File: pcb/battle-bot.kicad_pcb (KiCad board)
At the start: 4 copper layers, 99.2 x 51.2 mm, 27 parts, among them U1 TPS5430DDA, U2 STM32G474VETx

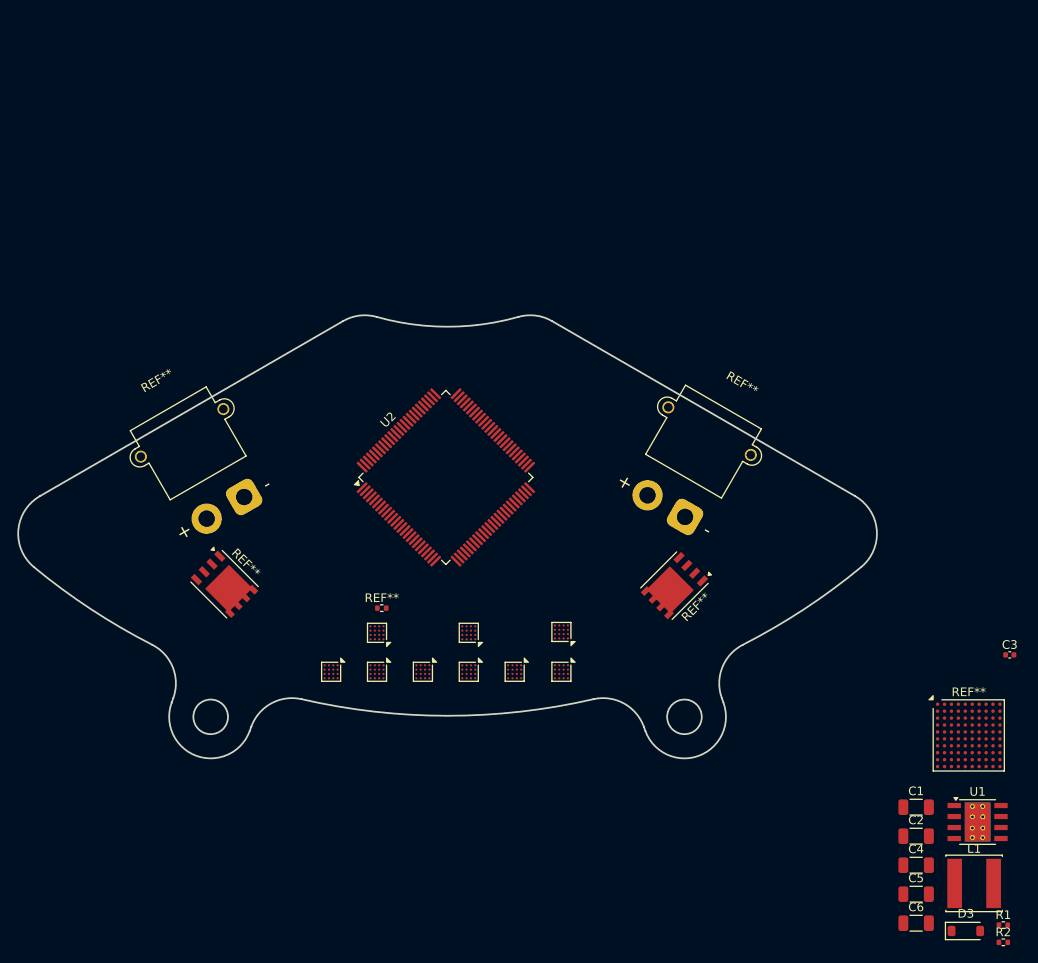
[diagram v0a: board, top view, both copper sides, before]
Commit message: Finish drivers
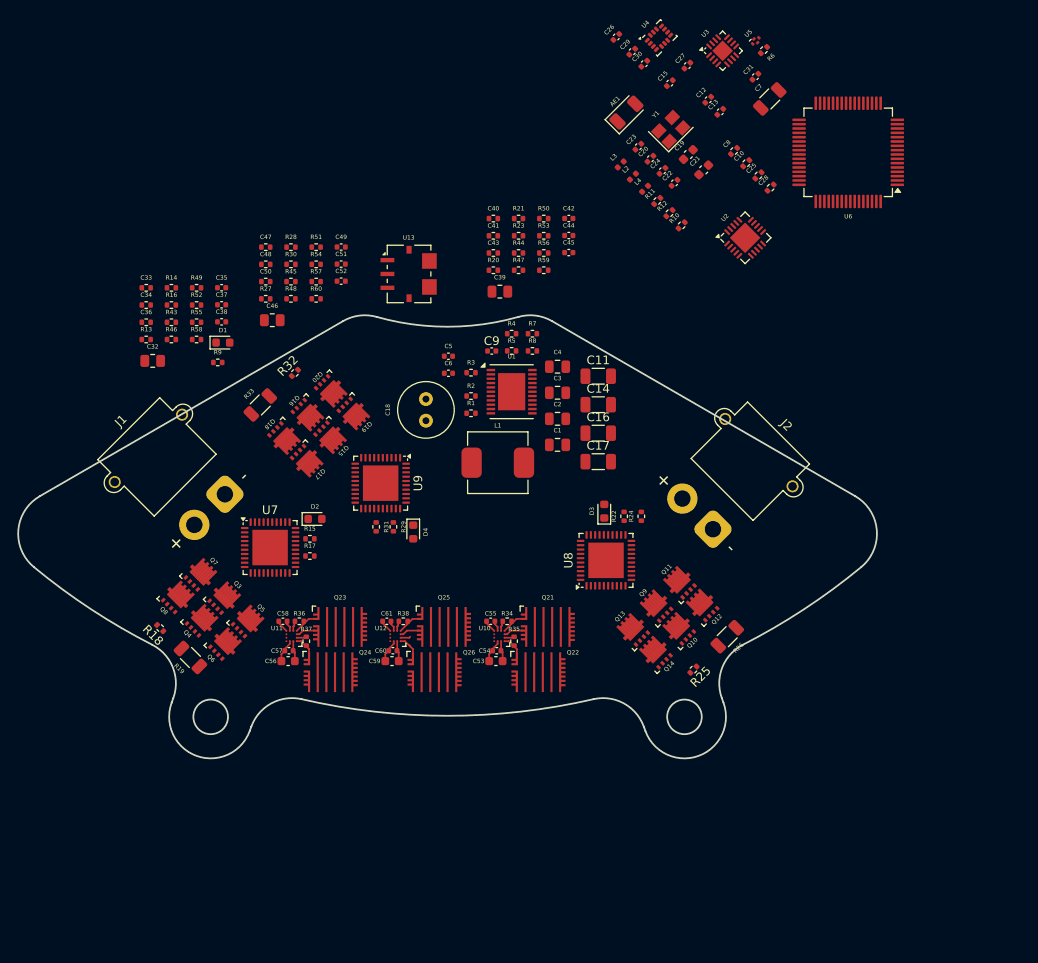
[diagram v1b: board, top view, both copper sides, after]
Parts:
- removed REF** (x9): BGA-16_1.92x1.92mm_Layout4x4_P0.5mm, Package_BGA:BGA-16_1.92x1.92mm_Layout4x4_P0.5mm
- removed REF** (x2): AMASS_XT30PW-M_1x02_P2.50mm_Horizontal, Connector_AMASS:AMASS_XT30PW-M_1x02_P2.50mm_Horizontal
- removed REF**: TFBGA-100_8x8mm_Layout10x10_P0.8mm, Package_BGA:TFBGA-100_8x8mm_Layout10x10_P0.8mm
- removed REF** (x2): PowerPAK_SO-8_Single, Package_SO:PowerPAK_SO-8_Single
- removed REF**: R_0402_1005Metric, Resistor_SMD:R_0402_1005Metric
- added AE1: Antenna, RF_Antenna:Johanson_2450AT18x100, F.Cu at (120.8, 7.26)
- added C10: 100n, Resistor_SMD:R_0402_1005Metric, F.Cu at (134.7, 13.1)
- added C11: 47u, Capacitor_SMD:C_1206_3216Metric, F.Cu at (117.6, 37.7)
- added C12: 10n, Capacitor_SMD:C_0402_1005Metric, F.Cu at (130.3, 5.78)
- added C13: 33n, Capacitor_SMD:C_0402_1005Metric, F.Cu at (131.7, 7.17)
- added C14: 47u, Capacitor_SMD:C_1206_3216Metric, F.Cu at (117.6, 41.0)
- added C15: 1n, Capacitor_SMD:C_0402_1005Metric, F.Cu at (125.9, 3.86)
- added C16: 47u, Capacitor_SMD:C_1206_3216Metric, F.Cu at (117.6, 44.3)
- added C17: 47u, Capacitor_SMD:C_1206_3216Metric, F.Cu at (117.6, 47.6)
- added C18: 220u, Capacitor_THT:C_Radial_D6.3mm_H7.0mm_P2.50mm, F.Cu at (97.7, 42.8)
- added C19: 2n2, Capacitor_SMD:C_0603_1608Metric, F.Cu at (128.0, 12.1)
- added C20: 12p, Capacitor_SMD:C_0402_1005Metric, F.Cu at (123.6, 12.6)
- added C21: 4p7, Capacitor_SMD:C_0603_1608Metric, F.Cu at (129.8, 13.9)
- added C22: 1p5, Capacitor_SMD:C_0402_1005Metric, F.Cu at (126.4, 15.4)
- added C23: 12p, Capacitor_SMD:C_0402_1005Metric, F.Cu at (122.2, 11.2)
- added C24: 1p, Capacitor_SMD:C_0402_1005Metric, F.Cu at (125.0, 14.0)
- added C25: 10u, Resistor_SMD:R_0402_1005Metric, F.Cu at (136.1, 14.5)
- added C26: 4u7, Capacitor_SMD:C_0402_1005Metric, F.Cu at (119.7, -1.48)
- added C27: 10n, Capacitor_SMD:C_0402_1005Metric, F.Cu at (127.9, 1.83)
- added C28: 220p, Resistor_SMD:R_0402_1005Metric, F.Cu at (137.5, 15.9)
- added C29: 100n, Capacitor_SMD:C_0402_1005Metric, F.Cu at (121.5, 0.22)
- added C30: 100n, Capacitor_SMD:C_0402_1005Metric, F.Cu at (122.9, 1.61)
- added C31: 0p3, Capacitor_SMD:C_0402_1005Metric, F.Cu at (135.8, 3.11)
- added C32: 22u, Resistor_SMD:R_0805_2012Metric, F.Cu at (66.1, 35.9)
- added C33: 1u, Resistor_SMD:R_0402_1005Metric, F.Cu at (65.4, 27.5)
- added C34: 1u, Resistor_SMD:R_0402_1005Metric, F.Cu at (65.4, 29.5)
- added C35: 100n, Capacitor_SMD:C_0402_1005Metric, F.Cu at (74.1, 27.5)
- added C36: 1u, Resistor_SMD:R_0402_1005Metric, F.Cu at (65.4, 31.5)
- added C37: 47n, Capacitor_SMD:C_0402_1005Metric, F.Cu at (74.1, 29.5)
- added C38: 100n, Capacitor_SMD:C_0402_1005Metric, F.Cu at (74.1, 31.4)
- added C39: 22u, Resistor_SMD:R_0805_2012Metric, F.Cu at (106.2, 27.9)
- added C40: 1u, Resistor_SMD:R_0402_1005Metric, F.Cu at (105.5, 19.5)
- added C41: 1u, Resistor_SMD:R_0402_1005Metric, F.Cu at (105.5, 21.5)
- added C42: 100n, Capacitor_SMD:C_0402_1005Metric, F.Cu at (114.2, 19.5)
- added C43: 1u, Resistor_SMD:R_0402_1005Metric, F.Cu at (105.5, 23.5)
- added C44: 47n, Capacitor_SMD:C_0402_1005Metric, F.Cu at (114.2, 21.5)
- added C45: 100n, Capacitor_SMD:C_0402_1005Metric, F.Cu at (114.2, 23.4)
- added C46: 22u, Resistor_SMD:R_0805_2012Metric, F.Cu at (80.0, 31.2)
- added C47: 1u, Resistor_SMD:R_0402_1005Metric, F.Cu at (79.2, 22.8)
- added C48: 1u, Resistor_SMD:R_0402_1005Metric, F.Cu at (79.2, 24.8)
- added C49: 100n, Capacitor_SMD:C_0402_1005Metric, F.Cu at (87.9, 22.8)
- added C50: 1u, Resistor_SMD:R_0402_1005Metric, F.Cu at (79.2, 26.8)
- added C51: 47n, Capacitor_SMD:C_0402_1005Metric, F.Cu at (87.9, 24.8)
- added C52: 100n, Capacitor_SMD:C_0402_1005Metric, F.Cu at (87.9, 26.7)
- added C53: 10u, Capacitor_SMD:C_0603_1608Metric, F.Cu at (105.8, 70.6)
- added C54: 100n, Capacitor_SMD:C_0402_1005Metric, F.Cu at (105.9, 69.4)
- added C55: 220n, Capacitor_SMD:C_0402_1005Metric, F.Cu at (105.2, 66.0)
- added C56: 10u, Capacitor_SMD:C_0603_1608Metric, F.Cu at (81.8, 70.6)
- added C57: 100n, Capacitor_SMD:C_0402_1005Metric, F.Cu at (81.9, 69.4)
- added C58: 220n, Capacitor_SMD:C_0402_1005Metric, F.Cu at (81.2, 66.0)
- added C59: 10u, Capacitor_SMD:C_0603_1608Metric, F.Cu at (93.8, 70.6)
- added C60: 100n, Capacitor_SMD:C_0402_1005Metric, F.Cu at (93.9, 69.4)
- added C61: 220n, Capacitor_SMD:C_0402_1005Metric, F.Cu at (93.2, 66.0)
- added C7: 100u, Resistor_SMD:R_1206_3216Metric, F.Cu at (137.4, 5.69)
- added C8: 10u, Resistor_SMD:R_0402_1005Metric, F.Cu at (133.3, 11.7)
- added C9: 100n, Capacitor_SMD:C_0402_1005Metric, F.Cu at (105.3, 34.8)
- added D1: LEDG, LED_SMD:LED_0603_1608Metric, F.Cu at (74.2, 33.8)
- added D2: LEDR, LED_SMD:LED_0603_1608Metric, F.Cu at (84.9, 54.2)
- added D4: LEDR, LED_SMD:LED_0603_1608Metric, F.Cu at (96.2, 55.7)
- added J1: Conn_01x02_Pin, Connector_AMASS:AMASS_XT30PW-M_1x02_P2.50mm_Horizontal, F.Cu at (74.5, 51.3)
- added J2: Conn_01x02_Pin, Connector_AMASS:AMASS_XT30PW-M_1x02_P2.50mm_Horizontal, F.Cu at (130.9, 55.4)
- added L2: 2n7, Inductor_SMD:L_0402_1005Metric, F.Cu at (121.6, 14.7)
- added L3: 8n2, Inductor_SMD:L_0402_1005Metric, F.Cu at (120.2, 13.3)
- added L4: 3n9, Inductor_SMD:L_0402_1005Metric, F.Cu at (123.0, 16.1)
- added Q10: AON7544, User_Footprints:DFN3x3A_8L_EP1_P, F.Cu at (127.0, 66.9)
- added Q11: AON7544, User_Footprints:DFN3x3A_8L_EP1_P, F.Cu at (127.1, 61.6)
- added Q12: AON7544, User_Footprints:DFN3x3A_8L_EP1_P, F.Cu at (129.7, 64.2)
- added Q13: AON7544, User_Footprints:DFN3x3A_8L_EP1_P, F.Cu at (121.7, 67.0)
- added Q14: AON7544, User_Footprints:DFN3x3A_8L_EP1_P, F.Cu at (124.3, 69.6)
- added Q15: AON7544, User_Footprints:DFN3x3A_8L_EP1_P, F.Cu at (86.6, 44.8)
- added Q16: AON7544, User_Footprints:DFN3x3A_8L_EP1_P, F.Cu at (84.0, 42.1)
- added Q17: AON7544, User_Footprints:DFN3x3A_8L_EP1_P, F.Cu at (83.9, 47.5)
- added Q18: AON7544, User_Footprints:DFN3x3A_8L_EP1_P, F.Cu at (81.3, 44.8)
- added Q19: AON7544, User_Footprints:DFN3x3A_8L_EP1_P, F.Cu at (89.3, 42.0)
- added Q20: AON7544, User_Footprints:DFN3x3A_8L_EP1_P, F.Cu at (86.7, 39.4)
- added Q21: GANE3R9, User_Footprints:GANE3R9, F.Cu at (111.8, 66.7)
- added Q22: GANE3R9, User_Footprints:GANE3R9, F.Cu at (110.7, 71.9)
- added Q23: GANE3R9, User_Footprints:GANE3R9, F.Cu at (87.8, 66.7)
- added Q24: GANE3R9, User_Footprints:GANE3R9, F.Cu at (86.7, 71.9)
- added Q25: GANE3R9, User_Footprints:GANE3R9, F.Cu at (99.8, 66.7)
- added Q26: GANE3R9, User_Footprints:GANE3R9, F.Cu at (98.7, 71.9)
- added Q3: AON7544, User_Footprints:DFN3x3A_8L_EP1_P, F.Cu at (74.4, 63.4)
- added Q4: AON7544, User_Footprints:DFN3x3A_8L_EP1_P, F.Cu at (71.8, 66.0)
- added Q5: AON7544, User_Footprints:DFN3x3A_8L_EP1_P, F.Cu at (77.1, 66.1)
- added Q6: AON7544, User_Footprints:DFN3x3A_8L_EP1_P, F.Cu at (74.5, 68.7)
- added Q7: AON7544, User_Footprints:DFN3x3A_8L_EP1_P, F.Cu at (71.7, 60.7)
- added Q8: AON7544, User_Footprints:DFN3x3A_8L_EP1_P, F.Cu at (69.0, 63.3)
- added Q9: AON7544, User_Footprints:DFN3x3A_8L_EP1_P, F.Cu at (124.4, 64.3)
- added R10: 1k, Resistor_SMD:R_0402_1005Metric, F.Cu at (127.2, 20.3)
- added R11: 1k, Resistor_SMD:R_0402_1005Metric, F.Cu at (124.4, 17.5)
- added R12: 22k, Resistor_SMD:R_0402_1005Metric, F.Cu at (125.8, 18.9)
- added R13: 47k, Resistor_SMD:R_0402_1005Metric, F.Cu at (65.4, 33.5)
- added R14: 1k, Resistor_SMD:R_0402_1005Metric, F.Cu at (68.3, 27.5)
- added R15: 510k, Resistor_SMD:R_0402_1005Metric, F.Cu at (84.3, 56.5)
- added R16: 47k, Resistor_SMD:R_0402_1005Metric, F.Cu at (68.3, 29.5)
- added R17: 510k, Resistor_SMD:R_0402_1005Metric, F.Cu at (84.3, 58.5)
- added R18: R, Resistor_SMD:R_0402_1005Metric, F.Cu at (67.0, 66.8)
- added R19: 2m, Resistor_SMD:R_1206_3216Metric, F.Cu at (70.5, 70.2)
- added R20: 47k, Resistor_SMD:R_0402_1005Metric, F.Cu at (105.5, 25.5)
- added R21: 1k, Resistor_SMD:R_0402_1005Metric, F.Cu at (108.4, 19.5)
- added R22: 510k, Resistor_SMD:R_0402_1005Metric, F.Cu at (120.6, 53.9)
- added R23: 47k, Resistor_SMD:R_0402_1005Metric, F.Cu at (108.4, 21.5)
- added R24: 510k, Resistor_SMD:R_0402_1005Metric, F.Cu at (122.6, 53.9)
- added R25: R, Resistor_SMD:R_0402_1005Metric, F.Cu at (128.6, 71.6)
- added R26: 2m, Resistor_SMD:R_1206_3216Metric, F.Cu at (132.5, 67.8)
- added R27: 47k, Resistor_SMD:R_0402_1005Metric, F.Cu at (79.2, 28.8)
- added R28: 1k, Resistor_SMD:R_0402_1005Metric, F.Cu at (82.1, 22.8)
- added R29: 510k, Resistor_SMD:R_0402_1005Metric, F.Cu at (93.9, 55.1)
- added R3: 100k, Resistor_SMD:R_0402_1005Metric, F.Cu at (102.9, 37.3)
- added R30: 47k, Resistor_SMD:R_0402_1005Metric, F.Cu at (82.1, 24.8)
- added R31: 510k, Resistor_SMD:R_0402_1005Metric, F.Cu at (92.0, 55.1)
- added R32: 10R, Resistor_SMD:R_0402_1005Metric, F.Cu at (82.6, 37.3)
- added R33: 2m, Resistor_SMD:R_1206_3216Metric, F.Cu at (78.6, 41.0)
- added R34: 10R, Resistor_SMD:R_0402_1005Metric, F.Cu at (107.1, 66.0)
- added R35: 10R, Resistor_SMD:R_0402_1005Metric, F.Cu at (107.9, 68.3)
- added R36: 10R, Resistor_SMD:R_0402_1005Metric, F.Cu at (83.1, 66.0)
- added R37: 10R, Resistor_SMD:R_0402_1005Metric, F.Cu at (83.9, 68.3)
- added R38: 10R, Resistor_SMD:R_0402_1005Metric, F.Cu at (95.1, 66.0)
- added R4: 100k, Resistor_SMD:R_0402_1005Metric, F.Cu at (107.6, 32.8)
- added R43: 10R, Resistor_SMD:R_0402_1005Metric, F.Cu at (68.3, 31.5)
- added R44: 10R, Resistor_SMD:R_0402_1005Metric, F.Cu at (108.4, 23.5)
- added R45: 10R, Resistor_SMD:R_0402_1005Metric, F.Cu at (82.1, 26.8)
- added R46: 10R, Resistor_SMD:R_0402_1005Metric, F.Cu at (68.3, 33.5)
- added R47: 10R, Resistor_SMD:R_0402_1005Metric, F.Cu at (108.4, 25.5)
- added R48: 10R, Resistor_SMD:R_0402_1005Metric, F.Cu at (82.1, 28.8)
- added R49: 10R, Resistor_SMD:R_0402_1005Metric, F.Cu at (71.2, 27.5)
- added R5: 15k, Resistor_SMD:R_0402_1005Metric, F.Cu at (107.6, 34.8)
- added R50: 10R, Resistor_SMD:R_0402_1005Metric, F.Cu at (111.3, 19.5)
- added R51: 10R, Resistor_SMD:R_0402_1005Metric, F.Cu at (85.0, 22.8)
- added R52: 10R, Resistor_SMD:R_0402_1005Metric, F.Cu at (71.2, 29.5)
- added R53: 10R, Resistor_SMD:R_0402_1005Metric, F.Cu at (111.3, 21.5)
- added R54: 10R, Resistor_SMD:R_0402_1005Metric, F.Cu at (85.0, 24.8)
- added R55: 10R, Resistor_SMD:R_0402_1005Metric, F.Cu at (71.2, 31.5)
- added R56: 10R, Resistor_SMD:R_0402_1005Metric, F.Cu at (111.3, 23.5)
- added R57: 10R, Resistor_SMD:R_0402_1005Metric, F.Cu at (85.0, 26.8)
- added R58: 10R, Resistor_SMD:R_0402_1005Metric, F.Cu at (71.2, 33.5)
- added R59: 10R, Resistor_SMD:R_0402_1005Metric, F.Cu at (111.3, 25.5)
- added R6: 22k, Resistor_SMD:R_0402_1005Metric, F.Cu at (136.7, 0.04)
- added R60: 10R, Resistor_SMD:R_0402_1005Metric, F.Cu at (85.0, 28.8)
- added R7: 10k, Resistor_SMD:R_0402_1005Metric, F.Cu at (110.0, 32.8)
- added R8: 100k, Resistor_SMD:R_0402_1005Metric, F.Cu at (110.0, 34.8)
- added R9: 1k, Resistor_SMD:R_0402_1005Metric, F.Cu at (73.7, 36.1)
- added U10: LMG1205, User_Footprints:LMG1205, F.Cu at (106.2, 67.7)
- added U11: LMG1205, User_Footprints:LMG1205, F.Cu at (82.2, 67.7)
- added U12: LMG1205, User_Footprints:LMG1205, F.Cu at (94.2, 67.7)
- added U13: ACS780xLRTR-100B, Sensor_Current:Allegro_PSOF-7_4.8x6.4mm_P1.60mm, F.Cu at (95.7, 25.9)
- added U3: AT2401C, Package_DFN_QFN:QFN-16-1EP_3x3mm_P0.5mm_EP1.7x1.7mm, F.Cu at (132.0, 0.12)
- added U4: ICM-42688-P, Package_LGA:LGA-14_3x2.5mm_P0.5mm_LayoutBorder3x4y, F.Cu at (124.6, -1.38)
- added U5: LFL152G45TC1A219, User_Footprints:LFL152G45TC1A219, F.Cu at (135.8, -1.03)
- added U6: STM32G431RBTx, Package_QFP:LQFP-64_10x10mm_P0.5mm, F.Cu at (146.5, 11.8)
- added U7: DRV8323H, Package_DFN_QFN:HVQFN-40-1EP_6x6mm_P0.5mm_EP4.1x4.1mm, F.Cu at (79.7, 57.5)
- added U8: DRV8323H, Package_DFN_QFN:HVQFN-40-1EP_6x6mm_P0.5mm_EP4.1x4.1mm, F.Cu at (118.5, 59.0)
- added U9: DRV8323H, Package_DFN_QFN:HVQFN-40-1EP_6x6mm_P0.5mm_EP4.1x4.1mm, F.Cu at (92.5, 50.1)
- added Y1: 16MHz, Crystal:Crystal_SMD_3225-4Pin_3.2x2.5mm, F.Cu at (126.0, 9.21)
- C1, C2: footprint Capacitor_SMD:C_1206_3216Metric -> Capacitor_SMD:C_0805_2012Metric
- C3: value 10n -> 22u; footprint Capacitor_SMD:C_0402_1005Metric -> Capacitor_SMD:C_0805_2012Metric
- C4: value 47u -> 22u; footprint Capacitor_SMD:C_1206_3216Metric -> Capacitor_SMD:C_0805_2012Metric
- C5, C6: value 47u -> 1u; footprint Capacitor_SMD:C_1206_3216Metric -> Capacitor_SMD:C_0402_1005Metric
- D3: value B5819W -> LEDR; footprint Diode_SMD:D_SOD-123 -> LED_SMD:LED_0603_1608Metric
- L1: value 15u -> 1u; footprint Inductor_SMD:L_Changjiang_FNR6020S -> Inductor_SMD:L_Changjiang_FXL0630
- R1: value R -> 22k
- R2: value R -> 10k
- U1: value TPS5430DDA -> TPS53319; footprint Package_SO:TI_SO-PowerPAD-8_ThermalVias -> Package_DFN_QFN:DFN-22-1EP_5x6mm_P0.5mm_EP3.14x4.3mm
- U2: value STM32G474VETx -> nRF24L01P; footprint Package_QFP:LQFP-100_14x14mm_P0.5mm -> Package_DFN_QFN:QFN-20-1EP_4x4mm_P0.5mm_EP2.5x2.5mm
- moved R2 88.1 mm to (102.9, 40.0)
- moved R1 85.3 mm to (102.9, 42.0)
- moved C6 83.4 mm to (100.3, 37.4)
- moved C5 82.3 mm to (100.3, 35.4)
- moved L1 73.4 mm to (106.0, 47.7)
- moved U1 73.3 mm to (107.6, 39.5)
- moved C4 70.9 mm to (112.9, 36.6)
- moved D3 64.0 mm to (118.3, 53.3), turned to 90 degrees
- moved C2 63.6 mm to (112.9, 42.6)
- moved C3 60.4 mm to (112.9, 39.6)
- moved C1 58.9 mm to (112.9, 45.6)
- moved U2 44.3 mm to (134.6, 21.7)
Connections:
- C1 pad 1: Net-(D1-K) -> VDD
- C2 pad 1: Net-(D1-K) -> VDD
- C3 pad 1: /BT -> VDD
- C3 pad 2: Net-(D3-K) -> GND
- C4 pad 1: +5V -> VDD
- C5 pad 1: +5V -> VDD
- C6 pad 1: +5V -> Net-(U1-VREG)
- D3 pad 2: GND -> +5V
- L1 pad 1: Net-(D3-K) -> Net-(C9-Pad1)
- R1 pad 1: +5V -> /REN
- R1 pad 2: /VSNS -> VDD
- R2 pad 1: /VSNS -> GND
- R2 pad 2: GND -> /REN
- U1 pad 1: /BT -> Net-(U1-VFB)
- U1 pad 2: unconnected-(U1-NC-Pad2) -> /REN
- U1 pad 3: unconnected-(U1-NC-Pad3) -> /PGD
- U1 pad 4: /VSNS -> Net-(U1-VBST)
- U1 pad 5: unconnected-(U1-EN-Pad5) -> GND
- U1 pad 6: GND -> Net-(C9-Pad1)
- U1 pad 7: Net-(D1-K) -> Net-(C9-Pad1)
- U1 pad 8: Net-(D3-K) -> Net-(C9-Pad1)
- U1 pad 9: GND -> Net-(C9-Pad1)
- U2 pad 1: unconnected-(U2-PE2-Pad1) -> /RCE
- U2 pad 10: unconnected-(U2-PF9-Pad10) -> /XC1
- U2 pad 11: unconnected-(U2-PF10-Pad11) -> /VPA
- U2 pad 12: unconnected-(U2-PF0-Pad12) -> Net-(U2-ANT1)
- U2 pad 13: unconnected-(U2-PF1-Pad13) -> Net-(U2-ANT2)
- U2 pad 14: unconnected-(U2-PG10-Pad14) -> GND
- U2 pad 15: unconnected-(U2-PC0-Pad15) -> +3V3
- U2 pad 16: unconnected-(U2-PC1-Pad16) -> Net-(U2-IREF)
- U2 pad 17: unconnected-(U2-PC2-Pad17) -> GND
- U2 pad 18: unconnected-(U2-PC3-Pad18) -> +3V3
- U2 pad 19: unconnected-(U2-PF2-Pad19) -> Net-(U2-DVDD)
- U2 pad 2: unconnected-(U2-PE3-Pad2) -> /RCS
- U2 pad 20: unconnected-(U2-PA0-Pad20) -> GND
- U2 pad 21: unconnected-(U2-PA1-Pad21) -> GND
- U2 pad 3: unconnected-(U2-PE4-Pad3) -> /CLK
- U2 pad 4: unconnected-(U2-PE5-Pad4) -> /MOSI
- U2 pad 5: unconnected-(U2-PE6-Pad5) -> /MISO
- U2 pad 6: unconnected-(U2-VBAT-Pad6) -> /RIRQ
- U2 pad 7: unconnected-(U2-PC13-Pad7) -> +3V3
- U2 pad 8: unconnected-(U2-PC14-Pad8) -> GND
- U2 pad 9: unconnected-(U2-PC15-Pad9) -> /XC2
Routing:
- net +5V: track 0.00 -> 8.11 mm
- net GND: track 0.00 -> 7.17 mm
- net /LargeMotor/LargeBridgeC/OUT: track 0.00 -> 3.77 mm
- net /LargeMotor/LargeBridgeB/OUT: track 0.00 -> 3.77 mm
- net /LargeMotor/LargeBridgeA/OUT: track 0.00 -> 3.77 mm
- net Net-(U12-HOL): track 0.00 -> 3.13 mm
- net Net-(U11-HOL): track 0.00 -> 3.13 mm
- net Net-(U10-HOL): track 0.00 -> 3.13 mm
- net Net-(U11-LOL): track 0.00 -> 2.94 mm
- net Net-(U12-LOL): track 0.00 -> 2.94 mm
- net Net-(U10-LOL): track 0.00 -> 2.94 mm
- net Net-(U11-HOH): track 0.00 -> 1.25 mm
- net Net-(U12-HOH): track 0.00 -> 1.25 mm
- net Net-(U10-HOH): track 0.00 -> 1.25 mm
- net Net-(U12-HB): track 0.00 -> 1.23 mm
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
